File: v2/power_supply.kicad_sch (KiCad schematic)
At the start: 30 parts, among them J1 Screw_Terminal_01x03, U14 LM7812, U8 LM7815, U9 LM7915

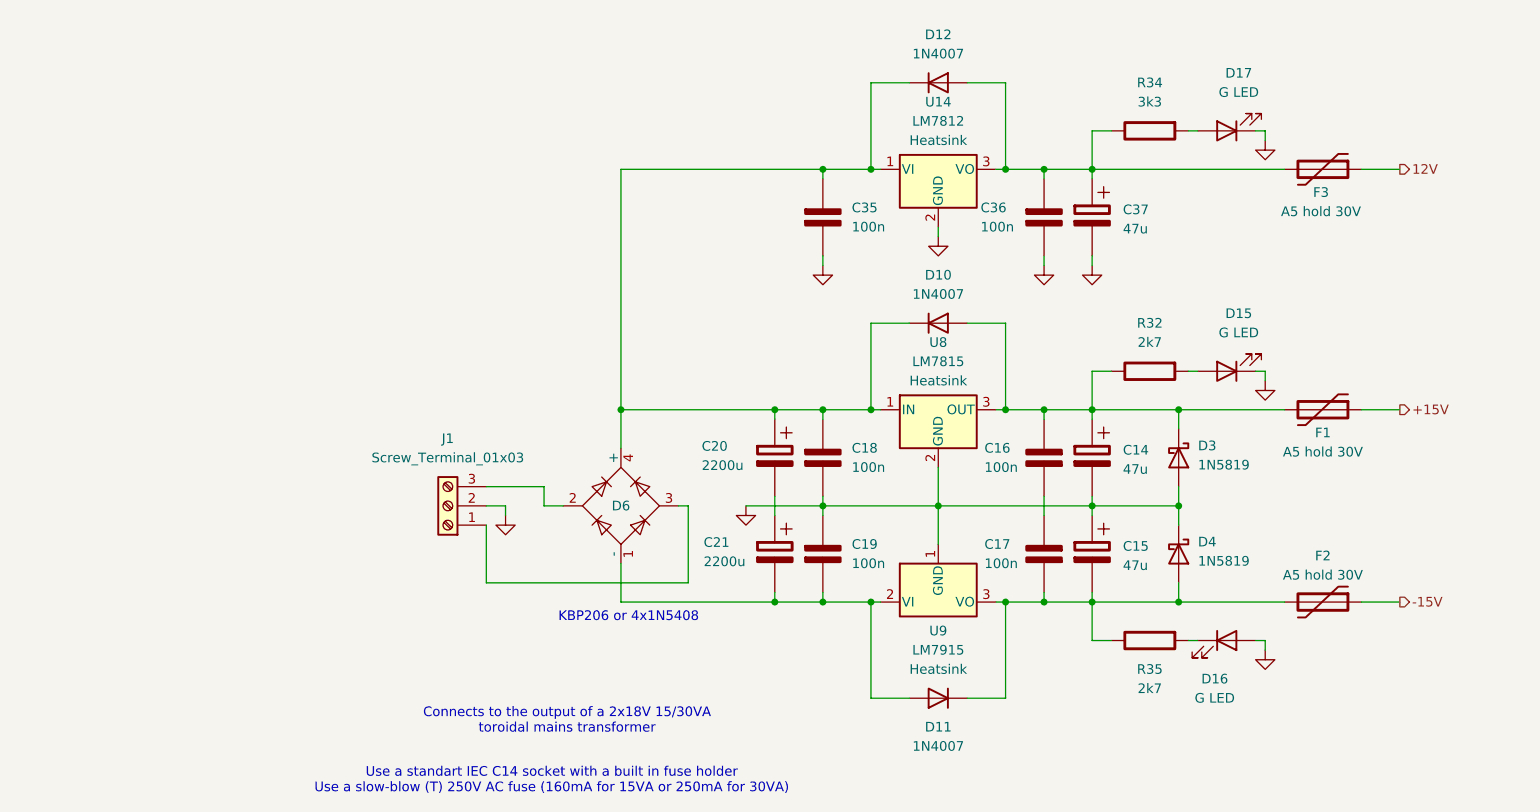
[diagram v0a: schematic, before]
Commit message: Finished, adding minure debug and production stuff, need to make PCB
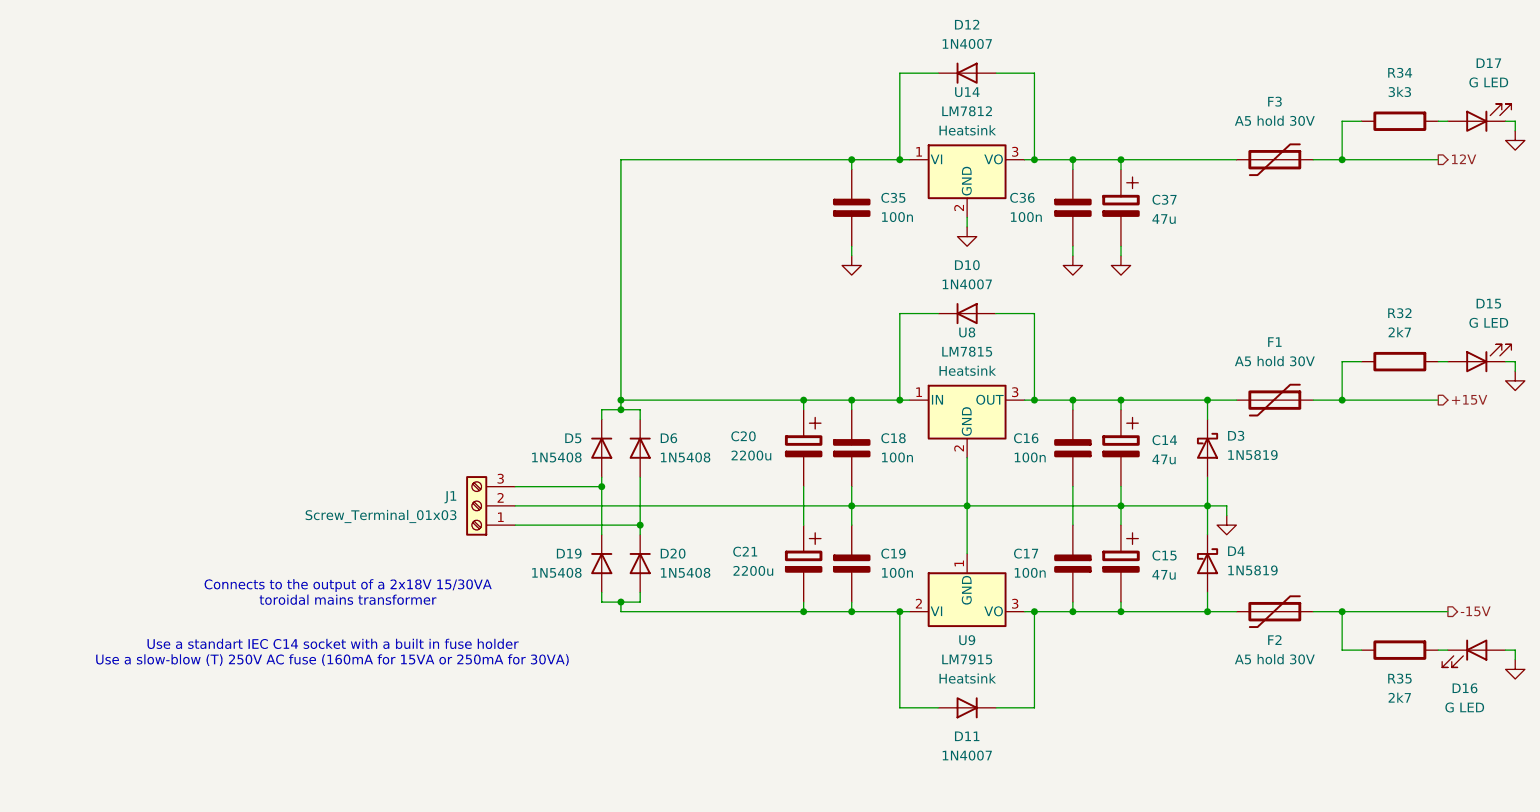
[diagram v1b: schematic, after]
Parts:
- removed D6: KBP206, Diode_THT:Diode_Bridge_19.0x3.5x10.0mm_P5.0mm, symbol Diode_Bridge:B40C2300-1500A
- added D19, D20, D5, D6: 1N5408, Diode_THT:D_DO-201AD_P15.24mm_Horizontal, symbol Diode:1N5408
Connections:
- net +15V: now also R32.
- net -15V: now also R35.
- net 12V: now also R34.
- net at C18., C20., C35.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: now also D5.1 (K), D6.1 (K)
- net at C19., C21., D11.2 (A)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: now also D19.2 (A), D20.2 (A)
- net at J1.1 (Pin_1): now also D20.1 (K), D6.2 (A)
- net at J1.3 (Pin_3): now also D19.1 (K), D5.2 (A)
- new net: C14., C16., D10.2 (A), D3.1 (K), F1., U8.3 (OUT)
- new net: C15., C17., D11.1 (K), D4.2 (A), F2., U9.3 (VO)
- new net: C36., C37., D12.2 (A), F3., U14.3 (VO)
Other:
- note removed: "KBP206 or 4x1N5408"
- moved on the sheet: C14, C15, C16, C17, C18, C19, C20, C21, C35, C36, C37, D10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
